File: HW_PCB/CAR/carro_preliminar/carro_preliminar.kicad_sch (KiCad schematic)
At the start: 25 parts, among them J1 V_Battery, J2 STLINK, J3 Puente H, J4 Puente_H2, J5 UART, J6 Servo_Motor, J7 NRF24_Con, SW1 SW_DPST_x2, U1 STM32F103C8Tx, U2 AMS1117-3.3, Y1 8MHz

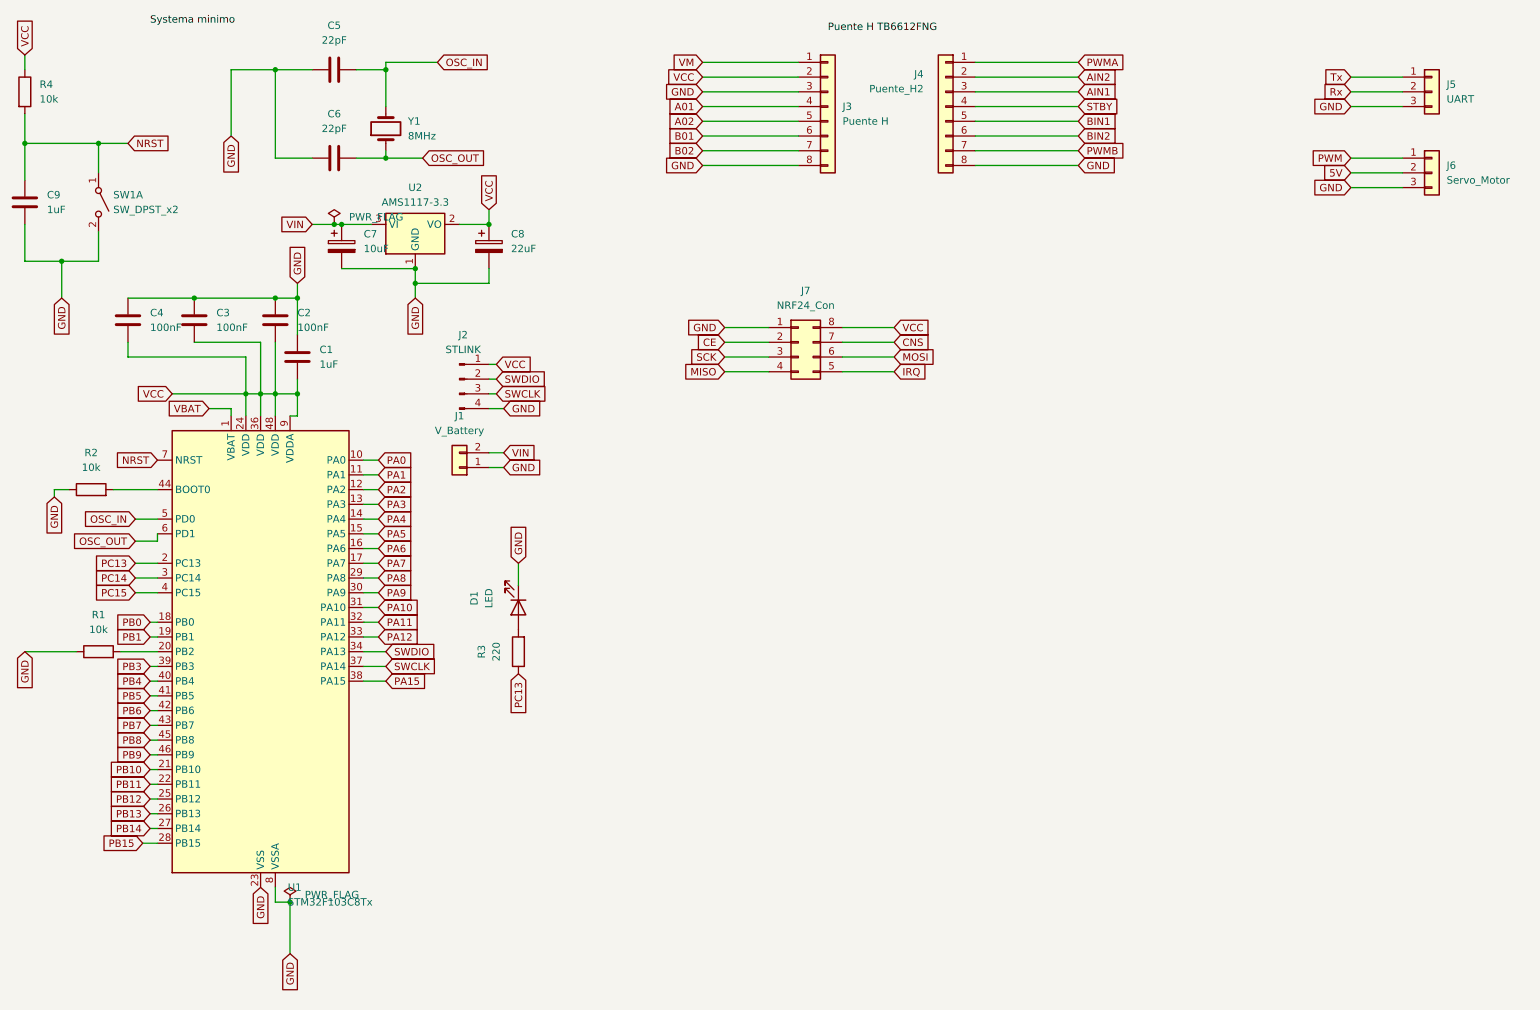
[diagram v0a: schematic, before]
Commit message: Carrito pcb, 25-02-26
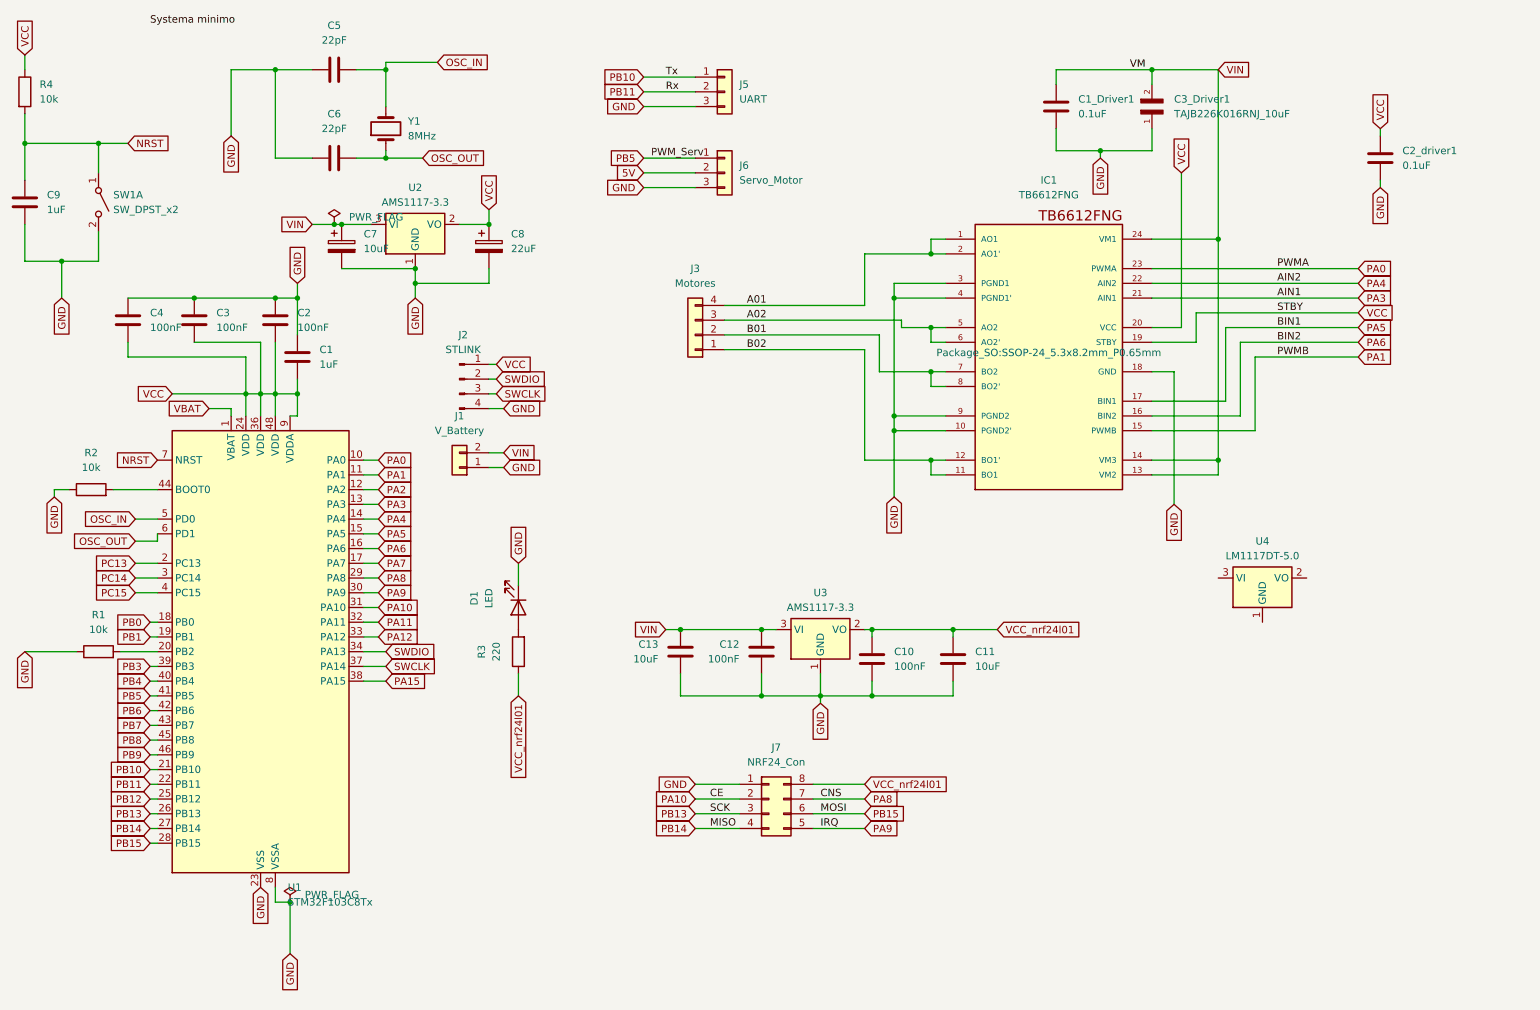
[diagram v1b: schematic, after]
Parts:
- removed J3: Puente H, Connector_PinHeader_2.54mm:PinHeader_1x08_P2.54mm_Vertical, symbol Connector_Generic:Conn_01x08
- removed J4: Puente_H2, Connector_PinHeader_2.54mm:PinHeader_1x08_P2.54mm_Vertical, symbol Connector_Generic:Conn_01x08
- added C10, C12: 100nF, Capacitor_SMD:C_0805_2012Metric_Pad1.18x1.45mm_HandSolder, symbol Device:C
- added C11, C13: 10uF, Capacitor_SMD:C_0805_2012Metric_Pad1.18x1.45mm_HandSolder, symbol Device:C
- added C1_Driver1, C2_driver1: 0.1uF, Capacitor_SMD:C_0805_2012Metric, symbol Device:C
- added C3_Driver1: TAJB226K016RNJ_10uF, TAJB226K016RNJ:CAPPC3528X210N, symbol TAJB226K016RNJ:TAJB226K016RNJ
- added IC1: TB6612FNG, Package_SO:SSOP-24_5.3x8.2mm_P0.65mm, symbol TB6612FNG:TB6612FNG
- added J3: Motores, Connector_PinHeader_2.54mm:PinHeader_1x04_P2.54mm_Vertical, symbol Connector_Generic:Conn_01x04
- added U3: AMS1117-3.3, Package_TO_SOT_SMD:SOT-223-3_TabPin2, symbol Regulator_Linear:AMS1117-3.3
- added U4: LM1117DT-5.0, Package_TO_SOT_SMD:TO-252-3_TabPin2, symbol Regulator_Linear:LM1117DT-5.0
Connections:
- net CE is gone; now on net PA10: J7.2 (Pin_2)
- net CNS is gone; now on net PA8: J7.7 (Pin_7)
- net IRQ is gone; now on net PA9: J7.5 (Pin_5)
- net MISO is gone; now on net PB14: J7.4 (Pin_4)
- net MOSI is gone; now on net PB15: J7.6 (Pin_6)
- net PWM is gone; now on net PB5: J6.1 (Pin_1)
- net Rx is gone; now on net PB11: J5.2 (Pin_2)
- net SCK is gone; now on net PB13: J7.3 (Pin_3)
- net Tx is gone; now on net PB10: J5.1 (Pin_1)
- net A01: now also IC1.1 (AO1), IC1.2 (AO1'), J3.4 (Pin_4)
- net A02: now also IC1.5 (AO2), IC1.6 (AO2'), J3.3 (Pin_3)
- net B01: now also IC1.7 (BO2), IC1.8 (BO2'), J3.2 (Pin_2)
- net B02: now also IC1.11 (BO1), IC1.12 (BO1'), J3.1 (Pin_1)
- net GND: now also C10.2, C11.2, C12.2, C13.2, C1_Driver1.2, C2_driver1.2, C3_Driver1.1, IC1.10 (PGND2'), IC1.18 (GND), IC1.3 (PGND1), IC1.4 (PGND1'), IC1.9 (PGND2), U3.1 (GND)
- net PA0: now also IC1.23 (PWMA)
- net PA1: now also IC1.15 (PWMB)
- net PA3: now also IC1.21 (AIN1)
- net PA4: now also IC1.22 (AIN2)
- net PA5: now also IC1.17 (BIN1)
- net PA6: now also IC1.16 (BIN2)
- net PC13: no longer R3.1
- net VCC: now also C2_driver1.1, IC1.19 (STBY), IC1.20 (VCC); no longer J7.8 (Pin_8)
- net VIN: now also C12.1, C13.1, C1_Driver1.1, C3_Driver1.2, IC1.13 (VM2), IC1.14 (VM3), IC1.24 (VM1), U3.3 (VI)
- new net VCC_nrf24l01: C10.1, C11.1, J7.8 (Pin_8), R3.1, U3.2 (VO)
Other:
- moved on the sheet: J5, J6, J7
